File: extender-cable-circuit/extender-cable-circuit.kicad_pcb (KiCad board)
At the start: 4 copper layers, 64 x 86 mm, 80 parts, among them X3 24MHz

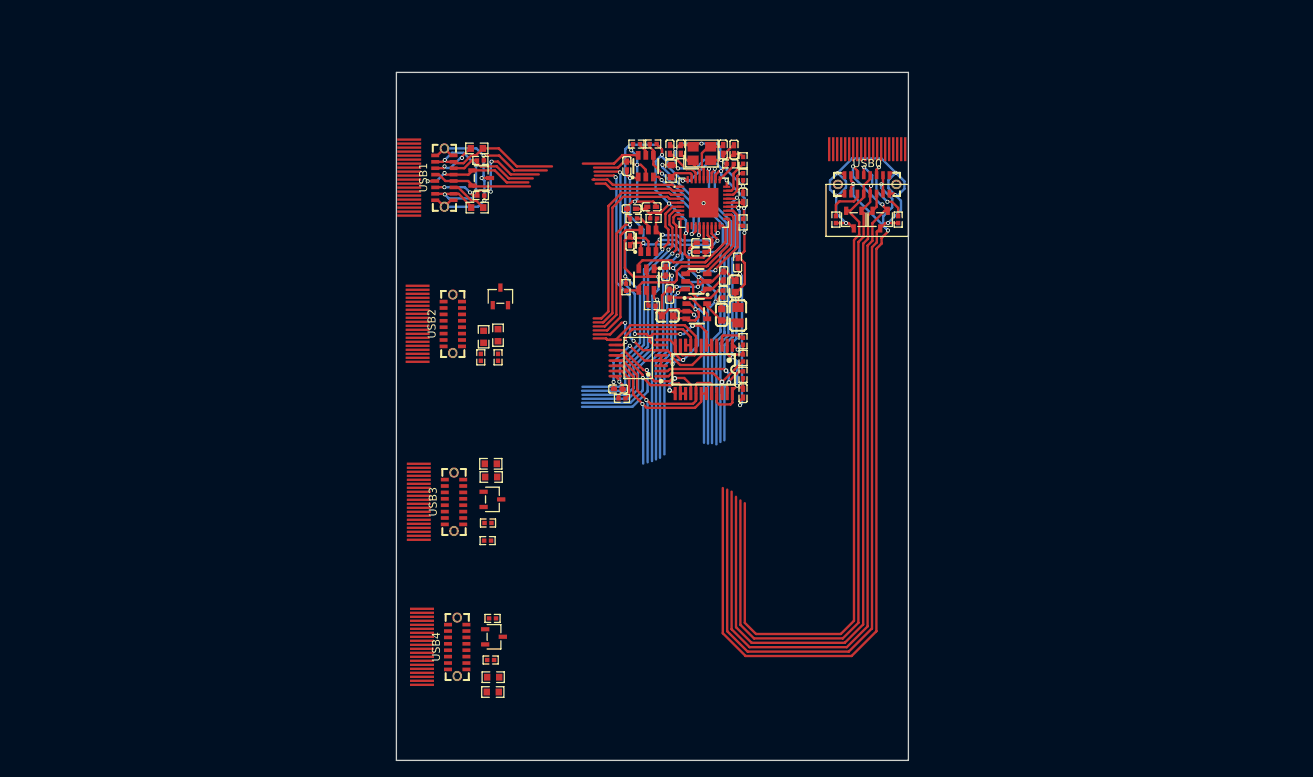
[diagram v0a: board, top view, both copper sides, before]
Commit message: Work on cable outline, and almost finish wiring.
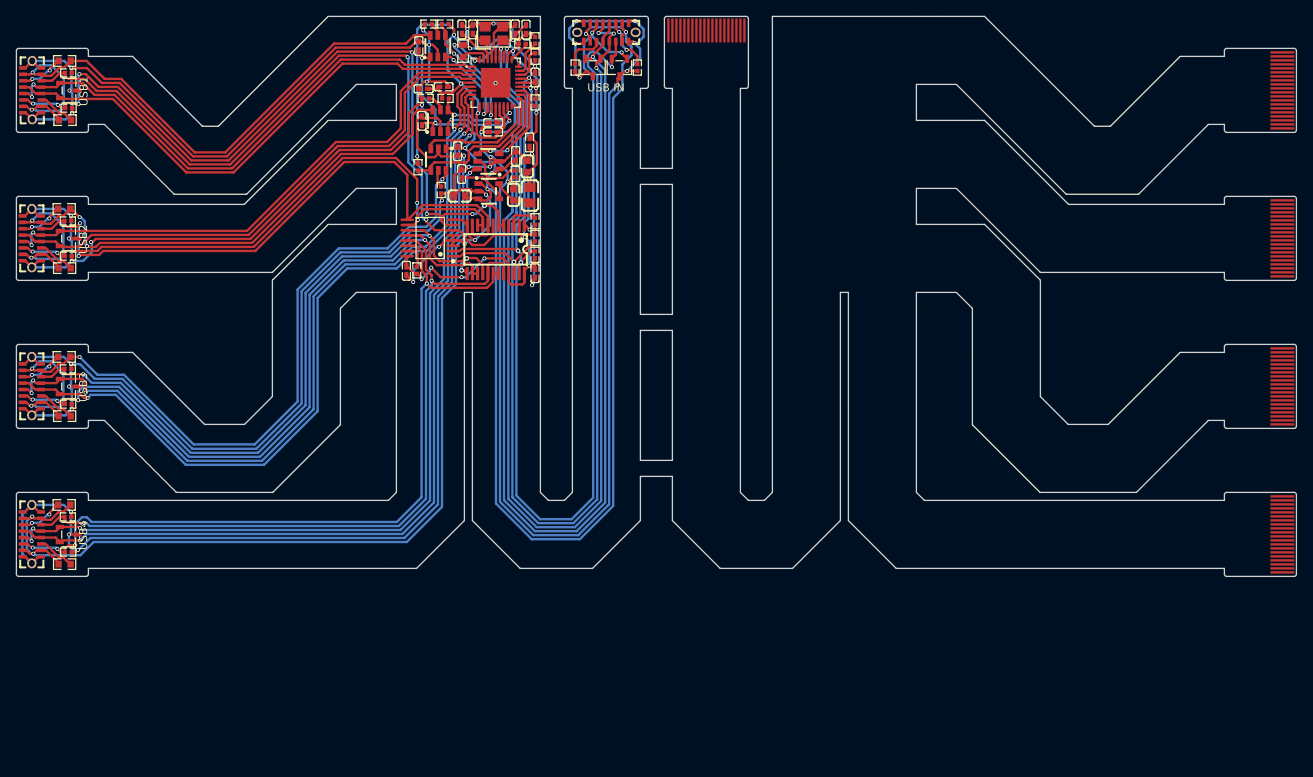
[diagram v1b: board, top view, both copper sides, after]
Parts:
- moved FPC1 109.7 mm to (210.8, 59.2), turned to -90 degrees
- moved FPC3 108.9 mm to (210.8, 96.2), turned to -90 degrees
- moved FPC2 108.6 mm to (210.8, 77.8), turned to -90 degrees
- moved FPC4 108.5 mm to (210.8, 114.8), turned to -90 degrees
- moved R20 58.4 mm to (58.5, 111.1)
- moved R18 56.5 mm to (58.5, 74.1), turned to 0 degrees
- moved R98 55.9 mm to (58.9, 94.1), turned to 180 degrees
- moved R99 55.8 mm to (58.9, 112.6)
- moved R81 55.4 mm to (58.5, 118.5)
- moved R104 55.2 mm to (59.0, 80.0), turned to 180 degrees
- moved R105 55.1 mm to (59.0, 98.5), turned to 180 degrees
- moved USB4 55.0 mm to (54.4, 114.7)
- moved R19 55.0 mm to (58.5, 92.6), turned to 0 degrees
- moved D16 54.8 mm to (59.0, 96.3)
- moved USB3 54.7 mm to (54.4, 96.2)
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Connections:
- FPC0 pad 1: GND -> VCC
- FPC0 pad 10: GND -> VCC
- FPC0 pad 11: VCC -> GND
- FPC0 pad 12: VCC -> GND
- FPC0 pad 13: VCC -> GND
- FPC0 pad 14: VCC -> GND
- FPC0 pad 15: VCC -> GND
- FPC0 pad 16: VCC -> GND
- FPC0 pad 17: VCC -> GND
- FPC0 pad 18: VCC -> GND
- FPC0 pad 19: VCC -> GND
- FPC0 pad 2: GND -> VCC
- FPC0 pad 20: VCC -> GND
- FPC0 pad 3: GND -> VCC
- FPC0 pad 4: GND -> VCC
- FPC0 pad 5: GND -> VCC
- FPC0 pad 6: GND -> VCC
- FPC0 pad 7: GND -> VCC
- FPC0 pad 8: GND -> VCC
- FPC0 pad 9: GND -> VCC
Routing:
- net GND: track 418.2 -> 689.8 mm, vias 36 -> 47
- net /servo-usb-connector3/VBUSx: track 22.1 -> 116.1 mm, vias 1 -> 3
- net /servo-usb-connector2/VBUSx: track 21.0 -> 102.1 mm, vias 1 -> 4
- net SERVO4_NRST: track 23.8 -> 99.2 mm, vias 1 -> 4
- net USBDN4_D-: track 33.0 -> 108.3 mm, vias 1 -> 4
- net USBDN4_D+: track 31.4 -> 106.5 mm, vias 1 -> 2
- net SERVO4_BOOT0: track 26.8 -> 97.7 mm, vias 1 -> 2
- net USBDN3_D-: track 31.4 -> 100.4 mm, vias 1 -> 4
- net SERVO3_NRST: track 21.6 -> 88.2 mm, vias 1 -> 4
- net USBDN3_D+: track 31.6 -> 97.7 mm, vias 1 -> 2
- net /servo-usb-connector1/VBUSx: track 17.1 -> 82.9 mm, vias 0 -> 4
- net SERVO3_BOOT0: track 27.3 -> 89.6 mm, vias 3 -> 4
- net SERVO2_BOOT0: track 19.5 -> 79.1 mm, vias 0 -> 2
- net SERVO2_NRST: track 19.7 -> 74.0 mm, vias 2 -> 4
- net USBDN2_D-: track 25.2 -> 69.4 mm, vias 0 -> 2
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- removed copper zone on In2.Cu, net GND
- removed copper zone on In1.Cu, net VCC
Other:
- board size 64 x 86 mm -> 160 x 70 mm
- copper layers 4 -> 2
- board text added: "Stiffner 0.3mm total"
